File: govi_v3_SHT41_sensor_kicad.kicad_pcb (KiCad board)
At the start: 2 copper layers, 81 x 89 mm, 76 parts, among them J201 Conn_01x03, J202 2.54mm 4-Pin JST, J203 Conn_01x04, J401 7.62mm 2-Pin Screw Terminal, J501 7.62mm 2-Pin Screw Terminal, Q501 Q_PMOS_Depletion, Q701 FS8205A, SW201 SW_Push, U201 STM32F103C6Tx, U301 Ra-02, U501 CN3791, U601 TP4056-42-ESOP8-AMS, U701 DW01A, U801 TPS63031DSK, Y201 8 MHz

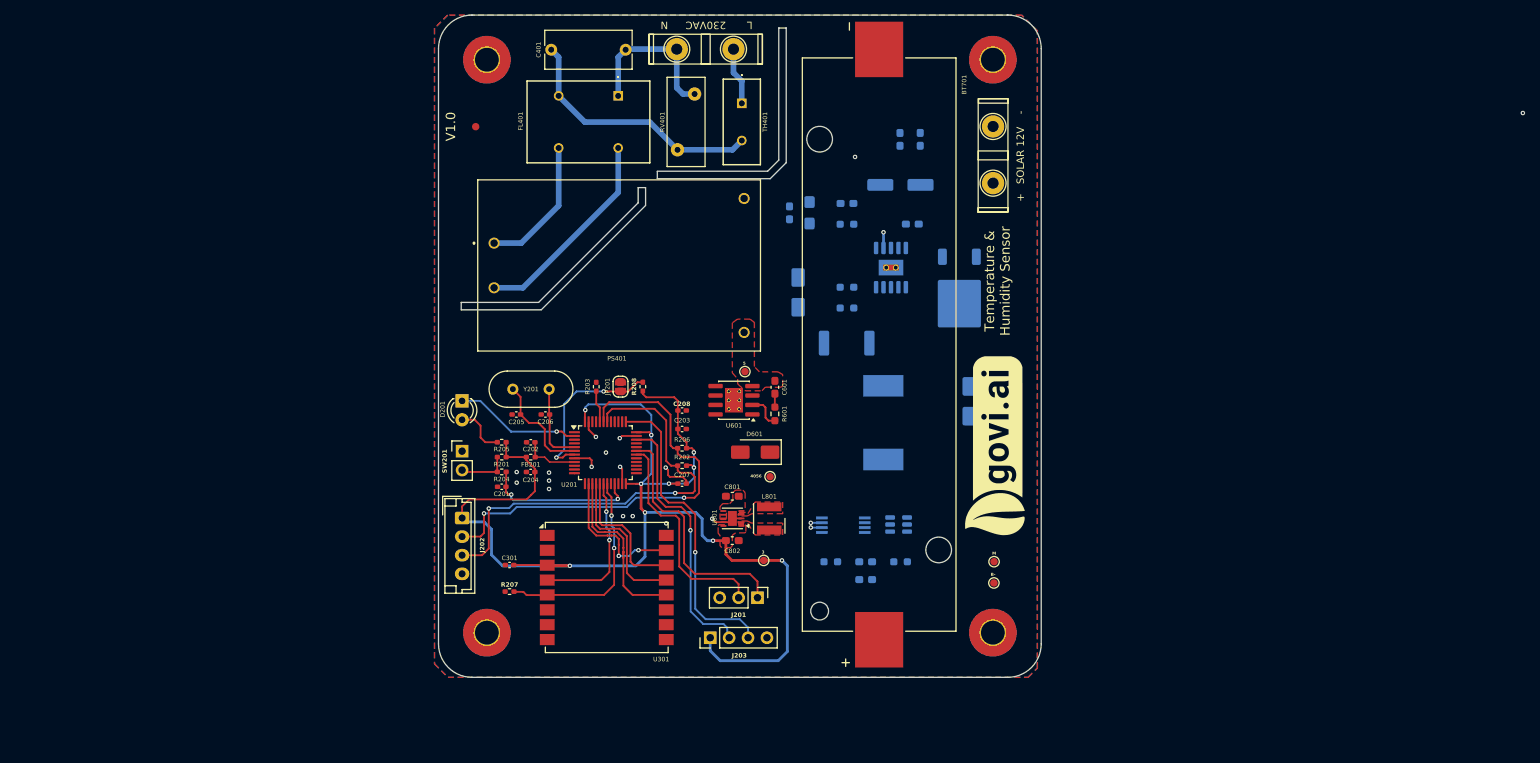
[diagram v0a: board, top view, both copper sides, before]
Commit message: "Routing done. DRC pending"
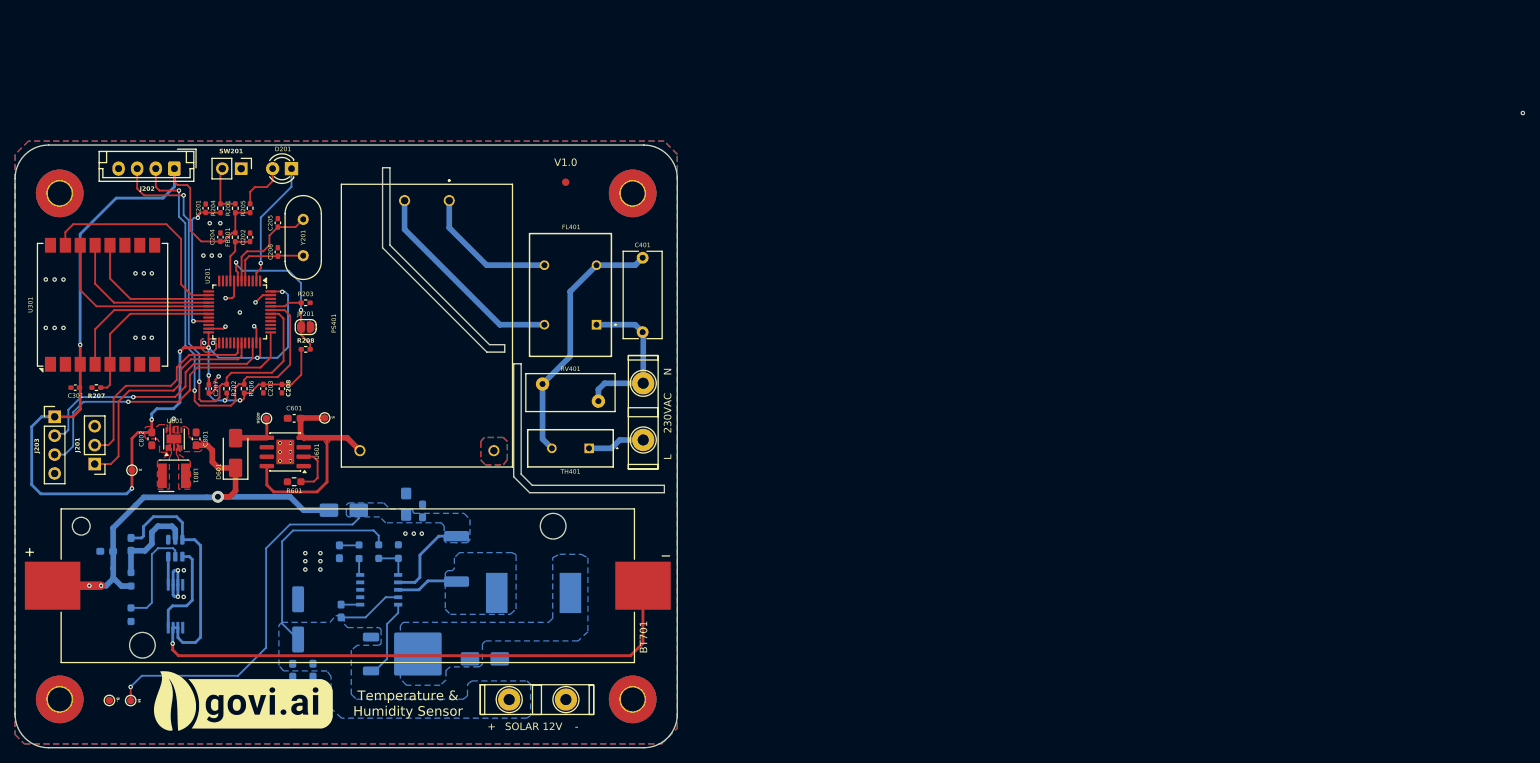
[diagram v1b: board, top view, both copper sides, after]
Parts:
- U501: footprint Package_SO:SSOP-10-1EP_3.9x4.9mm_P1mm_EP2.1x3.3mm_ThermalVias -> Package_SO:SSOP-10_3.9x4.9mm_P1.00mm
- moved H104 125.7 mm to (104.8, 134.3), turned to -90 degrees
- moved TP701 119.9 mm to (111.4, 134.5), turned to -90 degrees
- moved TP501 117.5 mm to (114.3, 134.5), turned to -90 degrees
- moved C502 110.5 mm to (136.1, 130.4), turned to -90 degrees
- moved G*** 107.3 mm to (129.5, 135.0), turned to 0 degrees
- moved C501 106.4 mm to (138.8, 130.4), turned to -90 degrees
- moved R702 103.4 mm to (114.3, 118.2), turned to 90 degrees
- moved C702 102.1 mm to (111.1, 114.4)
- moved C503 99.8 mm to (136.8, 123.6), turned to 90 degrees
- moved C701 98.8 mm to (114.3, 113.5), turned to 90 degrees
- moved H102 98.7 mm to (181.8, 134.3), turned to -90 degrees
- moved U701 97.3 mm to (120.3, 114.0), turned to 90 degrees
- moved J501 95.4 mm to (169.0, 134.4), turned to 0 degrees
- moved R701 94.3 mm to (114.3, 122.9), turned to -90 degrees
- moved J203 93.0 mm to (104.1, 96.3), turned to 0 degrees
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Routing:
- net Net-(BT701--): track 0.00 -> 107.1 mm, vias 0 -> 1
- net /3.3v_BuckBoost/IN+: track 0.52 -> 66.4 mm, vias 0 -> 3
- net Net-(D503-A): track 0.00 -> 63.0 mm, vias 0 -> 1
- net +12V: track 0.00 -> 38.5 mm
- net +5V: track 0.00 -> 31.8 mm
- net Net-(U701-CS): track 0.00 -> 14.1 mm
- net Net-(U701-OD): track 0.00 -> 13.0 mm
- net Net-(U701-VCC): track 0.00 -> 12.6 mm
- net Net-(Q501-G): track 0.00 -> 10.7 mm
- net /LoRa_Module_Ra-02/LoRa-NSS: track 19.6 -> 29.0 mm, vias 2 -> 0
- net Net-(U501-CSP): track 0.00 -> 8.39 mm
- net Net-(D601-A): track 0.21 -> 6.76 mm
- net /MCU/LoRa_INT: track 28.2 -> 22.6 mm, vias 2 -> 0
- net /LoRa_Module_Ra-02/LoRa-MOSI: track 18.8 -> 24.2 mm
- net Net-(U501-MPPT): track 0.00 -> 5.01 mm
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- added copper zone on B.Cu, net +12V
- added copper zone on B.Cu, net +3V3
- added copper zone on B.Cu, net Net-(D502-K)
- added copper zone on B.Cu, net Net-(D503-A)
- added copper zone on B.Cu, net Net-(U501-CSP)
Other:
- board size 81 x 89 mm -> 89 x 81 mm
